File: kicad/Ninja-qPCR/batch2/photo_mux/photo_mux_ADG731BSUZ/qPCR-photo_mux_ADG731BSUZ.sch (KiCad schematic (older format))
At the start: 17 parts

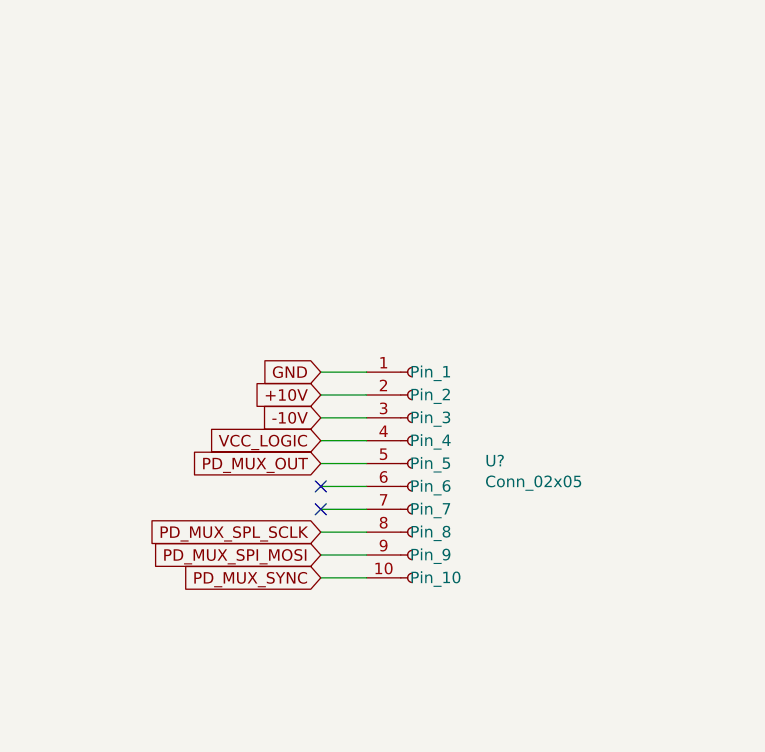
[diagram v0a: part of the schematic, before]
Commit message: sync
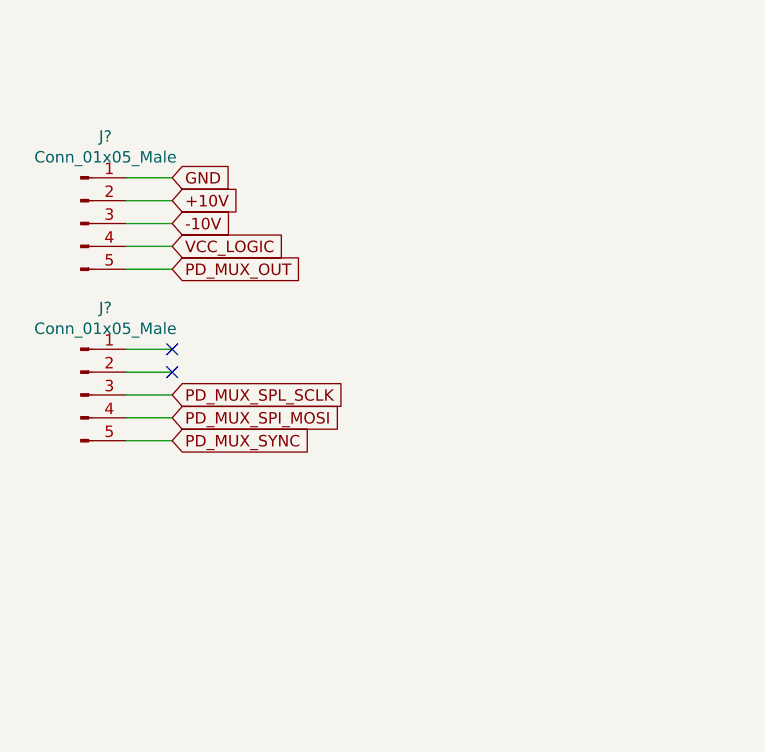
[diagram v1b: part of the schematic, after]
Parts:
- removed U?: Conn_02x05, symbol Ninja-qPCR:Conn_02x05
- added J? (x2): Conn_01x05_Male, symbol Connector:Conn_01x05_Male
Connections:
- net +10V: now also J?.2 (Pin_2)
- net -10V: now also J?.3 (Pin_3)
- net GND: now also J?.1 (Pin_1)
- net PD_MUX_OUT: now also J?.5 (Pin_5)
- net PD_MUX_SPI_MOSI: now also J?.4 (Pin_4)
- net PD_MUX_SPL_SCLK: now also J?.3 (Pin_3)
- net PD_MUX_SYNC: now also J?.5 (Pin_5)
- net VCC_LOGIC: now also J?.4 (Pin_4)
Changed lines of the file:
@@
 	1    0    0    -1
 $EndComp
-Text GLabel 1900 2050 0    50   Input ~ 0
-GND
-Text GLabel 1900 2150 0    50   Input ~ 0
+Text GLabel 1250 1200 2    50   Input ~ 0
+GND
+Text GLabel 1250 1300 2    50   Input ~ 0
 +10V
-Text GLabel 1900 2250 0    50   Input ~ 0
+Text GLabel 1250 1400 2    50   Input ~ 0
 -10V
-Text GLabel 1900 2350 0    50   Input ~ 0
+Text GLabel 1250 1500 2    50   Input ~ 0
 VCC_LOGIC
-Text GLabel 1900 2450 0    50   Input ~ 0
+Text GLabel 1250 1600 2    50   Input ~ 0
 PD_MUX_OUT
 Wire Wire Line
-	2100 2050 1900 2050
-Wire Wire Line
-	1900 2150 2100 2150
-Wire Wire Line
-	2100 2250 1900 2250
-Wire Wire Line
-	1900 2350 2100 2350
-Wire Wire Line
-	2100 2450 1900 2450
-Wire Wire Line
-	1900 2550 2100 2550
-Wire Wire Line
-	2100 2650 1900 2650
-Wire Wire Line
-	1900 2750 2100 2750
-Wire Wire Line
-	2100 2850 1900 2850
-$Comp
-L Ninja-qPCR:Conn_02x05 U?
-U 1 1 5F51FB4B
-P 2300 2050
-F 0 "U?" H 2619 1661 50  0000 L CNN
-F 1 "Conn_02x05" H 2619 1570 50  0000 L CNN
-F 2 "" H 2100 2150 50  0001 C CNN
-F 3 "" H 2100 2150 50  0001 C CNN
-	1    2300 2050
-	1    0    0    -1
-$EndComp
-Wire Wire Line
-	1900 2950 2100 2950
+	1050 1200 1250 1200
+Wire Wire Line
+	1250 1300 1050 1300
+Wire Wire Line
+	1050 1400 1250 1400
+Wire Wire Line
+	1250 1500 1050 1500
+Wire Wire Line
+	1050 1600 1250 1600
+Wire Wire Line
+	1250 1950 1050 1950
+Wire Wire Line
+	1050 2050 1250 2050
+Wire Wire Line
+	1250 2150 1050 2150
+Wire Wire Line
+	1050 2250 1250 2250
+Wire Wire Line
+	1250 2350 1050 2350
 $Comp
 L Ninja-qPCR:ADG731BSUZ U?
@@
 Wire Wire Line
 	6950 1050 6800 1050
-Text GLabel 1900 2750 0    50   Input ~ 0
+Text GLabel 1250 2150 2    50   Input ~ 0
 PD_MUX_SPL_SCLK
-Text GLabel 1900 2850 0    50   Input ~ 0
+Text GLabel 1250 2250 2    50   Input ~ 0
 PD_MUX_SPI_MOSI
-Text GLabel 1900 2950 0    50   Input ~ 0
+Text GLabel 1250 2350 2    50   Input ~ 0
 PD_MUX_SYNC
-NoConn ~ 1900 2550
+NoConn ~ 1250 1950
 Text GLabel 6800 1150 0    50   Input ~ 0
 PD_MUX_SPI_MOSI
@@
 Wire Wire Line
 	8550 4350 8700 4350
-NoConn ~ 1900 2650
+NoConn ~ 1250 2050
 Text GLabel 1750 4600 0    50   Input ~ 0
 +10V
@@
 Wire Wire Line
 	6950 5100 6750 5100
+$Comp
+L Connector:Conn_01x05_Male J?
+U 1 1 5F5948A2
+P 850 1400
+F 0 "J?" H 958 1781 50  0000 C CNN
+F 1 "Conn_01x05_Male" H 958 1690 50  0000 C CNN
+F 2 "" H 850 1400 50  0001 C CNN
+F 3 "~" H 850 1400 50  0001 C CNN
+	1    850  1400
+	1    0    0    -1
+$EndComp
+$Comp
+L Connector:Conn_01x05_Male J?
+U 1 1 5F5950CF
+P 850 2150
+F 0 "J?" H 958 2531 50  0000 C CNN
+F 1 "Conn_01x05_Male" H 958 2440 50  0000 C CNN
+F 2 "" H 850 2150 50  0001 C CNN
+F 3 "~" H 850 2150 50  0001 C CNN
+	1    850  2150
+	1    0    0    -1
+$EndComp
 $EndSCHEMATC
